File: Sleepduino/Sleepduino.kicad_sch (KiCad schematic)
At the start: 17 parts, among them J1 Barrel_Jack_Switch, J2 Conn_02x03_Counter_Clockwise, U1 ATmega328P-A, U2 ATmega16U2-A, U3 LP2985-3.3, U4 NCP1117-12_TO252, U5 RP2040, Y1 Crystal, Y2 Crystal

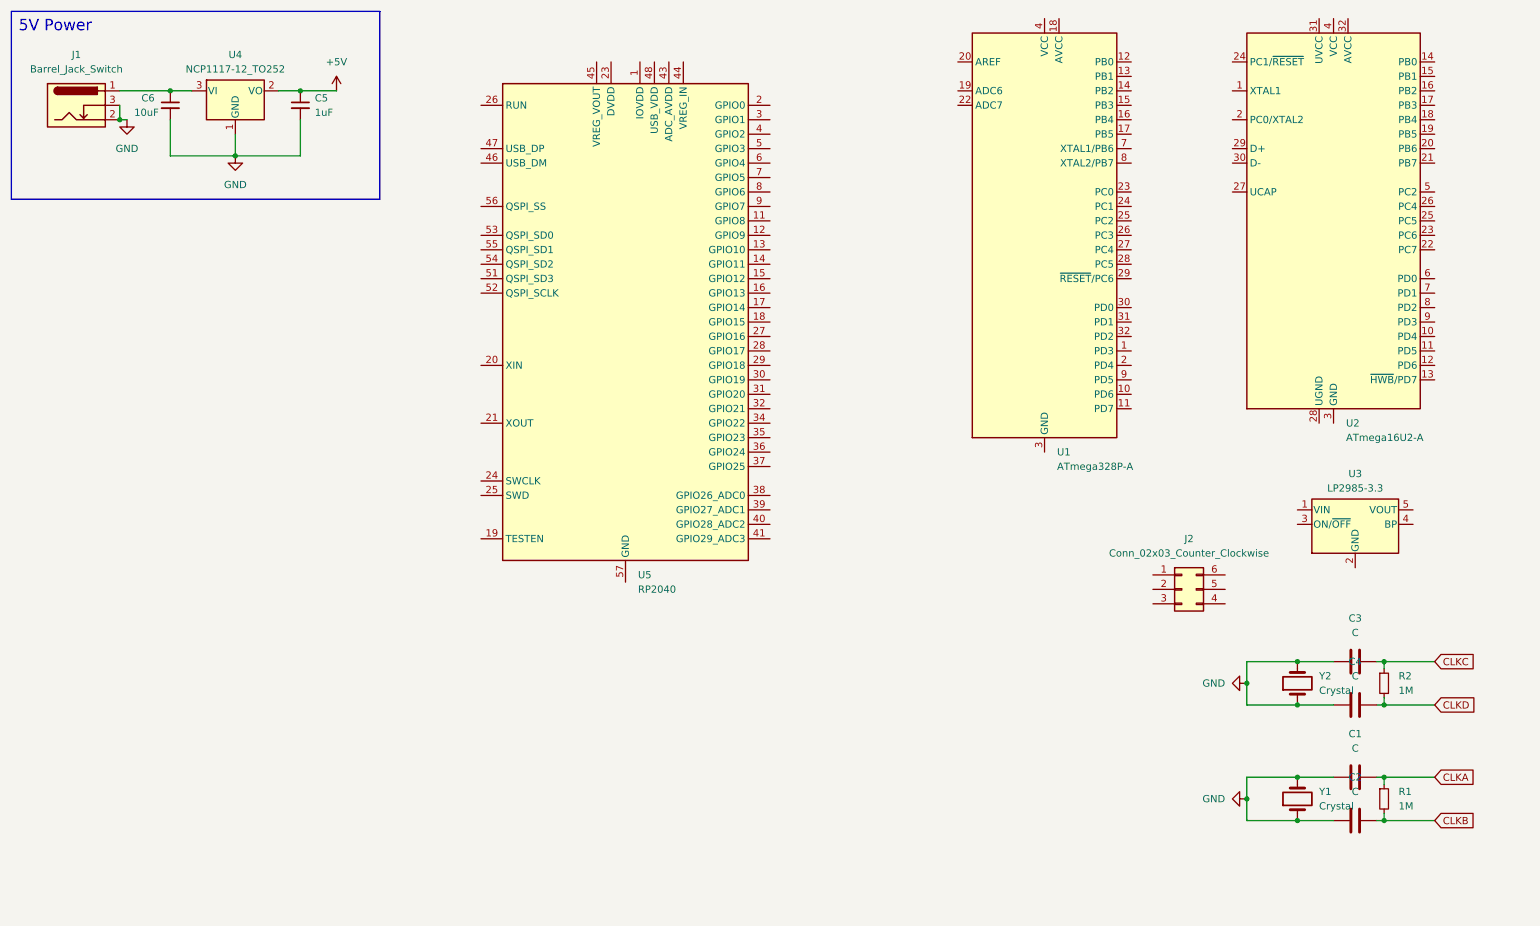
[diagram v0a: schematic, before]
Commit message: massive gains
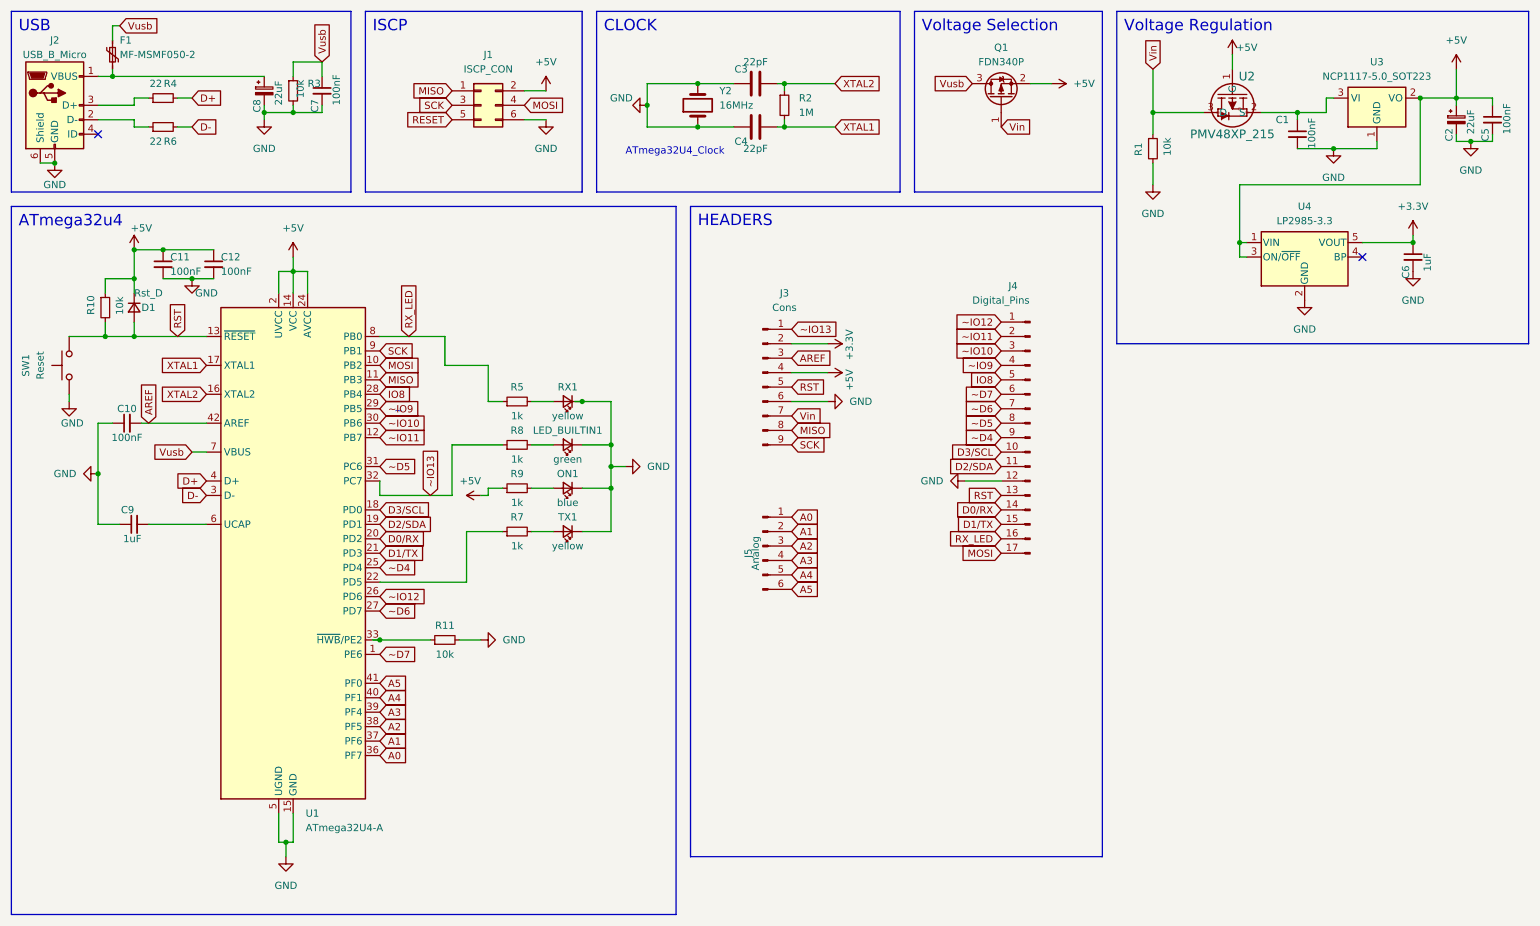
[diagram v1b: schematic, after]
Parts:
- removed C1, C2: C, Capacitor_SMD:C_0402_1005Metric, symbol Device:C
- removed J1: Barrel_Jack_Switch, symbol Connector:Barrel_Jack_Switch
- removed J2: Conn_02x03_Counter_Clockwise, symbol Connector_Generic:Conn_02x03_Counter_Clockwise
- removed U1: ATmega328P-A, Package_QFP:TQFP-32_7x7mm_P0.8mm, symbol MCU_Microchip_ATmega:ATmega328P-A
- removed U2: ATmega16U2-A, Package_QFP:TQFP-32_7x7mm_P0.8mm, symbol MCU_Microchip_ATmega:ATmega16U2-A
- removed U3: LP2985-3.3, Package_TO_SOT_SMD:SOT-23-5, symbol Regulator_Linear:LP2985-3.3
- removed U4: NCP1117-12_TO252, Package_TO_SOT_SMD:TO-252-2, symbol Regulator_Linear:NCP1117-12_TO252
- removed U5: RP2040, Package_DFN_QFN:QFN-56-1EP_7x7mm_P0.4mm_EP3.2x3.2mm, symbol MCU_RaspberryPi:RP2040
- removed Y1: Crystal, Crystal:Crystal_HC49-4H_Vertical, symbol Device:Crystal
- added C1, C10, C11, C12, C7: 100nF, Capacitor_SMD:C_0402_1005Metric, symbol Device:C_Small
- added C2, C8: 22uF, Capacitor_SMD:C_0402_1005Metric, symbol Device:C_Polarized_Small
- added C9: 1uF, Capacitor_SMD:C_0402_1005Metric, symbol Device:C_Small
- added D1: Rst_D, Diode_SMD:D_SOD-323, symbol Device:D_Small
- added F1: MF-MSMF050-2, Fuse:Fuse_1812_4532Metric, symbol Device:Polyfuse_Small
- added J1: ISCP_CON, Connector_PinHeader_2.54mm:PinHeader_2x03_P2.54mm_Vertical, symbol Connector_Generic:Conn_02x03_Odd_Even
- added J2: USB_B_Micro, Connector_USB:USB_Micro-B_Molex-105017-0001, symbol Connector:USB_B_Micro
- added J3: Cons, Connector_PinHeader_2.54mm:PinHeader_1x09_P2.54mm_Vertical, symbol Connector:Conn_01x09_Pin
- added J4: Digital_Pins, Connector_PinHeader_2.54mm:PinHeader_1x17_P2.54mm_Vertical, symbol Connector:Conn_01x17_Pin
- added J5: Analog, Connector_PinHeader_2.54mm:PinHeader_1x06_P2.54mm_Vertical, symbol Connector:Conn_01x06_Pin
- added LED_BUILTIN1: green, LED_SMD:LED_0603_1608Metric, symbol Device:LED_Small
- added ON1: blue, LED_SMD:LED_0603_1608Metric, symbol Device:LED_Small
- added Q1: FDN340P, Package_TO_SOT_SMD:SOT-23, symbol Transistor_FET:FDN340P
- added R10, R11, R3: 10k, Resistor_SMD:R_0402_1005Metric, symbol Device:R_Small
- added R4, R6: 22, Resistor_SMD:R_0402_1005Metric, symbol Device:R_Small
- added R5, R7, R8, R9: 1k, Resistor_SMD:R_0402_1005Metric, symbol Device:R_Small
- added RX1, TX1: yellow, LED_SMD:LED_0603_1608Metric, symbol Device:LED_Small
- added SW1: Reset, Button_Switch_SMD:SW_SPST_TL3342, symbol Switch:SW_Push
- added U1: ATmega32U4-A, Package_QFP:TQFP-44_10x10mm_P0.8mm, symbol MCU_Microchip_ATmega:ATmega32U4-A
- added U2: PMV48XP_215, footprints:TO-236_SOT23_NEX, symbol 2023-11-08_00-09-48:PMV48XP_215
- added U3: NCP1117-5.0_SOT223, Package_TO_SOT_SMD:SOT-223-3_TabPin2, symbol Regulator_Linear:NCP1117-5.0_SOT223
- added U4: LP2985-3.3, Package_TO_SOT_SMD:SOT-23-5, symbol Regulator_Linear:LP2985-3.3
- C3, C4: value C -> 22pF
- C5: value 1uF -> 100nF; footprint (none) -> Capacitor_SMD:C_0402_1005Metric
- C6: value 10uF -> 1uF; footprint (none) -> Capacitor_SMD:C_0402_1005Metric
- R1: value 1M -> 10k
- Y2: value Crystal -> 16MHz
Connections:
- net CLKB is gone; now on net GND: R1.2
- net +5V: now also C11.1, C12.1, C2.1, D1.1 (K), J1.2 (Pin_2), J3.4 (Pin_4), Q1.2 (S), R10.1, R9.1, U1.14 (VCC), U1.2 (UVCC), U1.24 (AVCC), U1.34 (VCC), U1.44 (AVCC), U2.1 (G), U3.2 (VO), U4.1 (VIN), U4.3 (ON/~{OFF})
- net GND: now also C1.2, C10.1, C11.2, C12.2, C2.2, C7.2, C8.2, C9.1, J1.6 (Pin_6), J2.5 (GND), J2.6 (Shield), J3.6 (Pin_6), J4.12 (Pin_12), LED_BUILTIN1.1 (K), ON1.1 (K), R11.2, R3.2, RX1.1 (K), SW1.1, TX1.1 (K), U1.15 (GND), U1.23 (GND), U1.35 (GND), U1.43 (GND), U1.5 (UGND), U3.1 (GND), U4.2 (GND)
- net +3.3V: now reaches C6.1
- net +3.3V: now also J3.2 (Pin_2), U4.5 (VOUT)
- net CLKA renamed Vin
- net Vin: now also J3.7 (Pin_7), Q1.1 (G), U2.3 (D)
- net CLKC renamed XTAL2
- net XTAL2: now also U1.16 (XTAL2)
- net CLKD renamed XTAL1
- net XTAL1: now also U1.17 (XTAL1)
- new net: R7.1, U1.22 (PD5)
- new net: R11.1, U1.33 (~{HWB}/PE2)
- new net: C9.2, U1.6 (UCAP)
- new net: C1.1, U2.2 (S), U3.3 (VI)
- new net: J2.3 (D+), R4.1
- new net: LED_BUILTIN1.2 (A), R8.2
- new net: R5.2, RX1.2 (A)
- new net: C8.1, F1.2, J2.1 (VBUS)
- new net: R7.2, TX1.2 (A)
- new net: J2.2 (D-), R6.1
- new net: ON1.2 (A), R9.2
- new net A0: J5.1 (Pin_1), U1.36 (PF7)
- new net A1: J5.2 (Pin_2), U1.37 (PF6)
- new net A2: J5.3 (Pin_3), U1.38 (PF5)
- new net A3: J5.4 (Pin_4), U1.39 (PF4)
- new net A4: J5.5 (Pin_5), U1.40 (PF1)
- new net A5: J5.6 (Pin_6), U1.41 (PF0)
- new net AREF: C10.2, J3.3 (Pin_3), U1.42 (AREF)
- new net D+: R4.2, U1.4 (D+)
- new net D-: R6.2, U1.3 (D-)
- new net D0/RX: J4.14 (Pin_14), U1.20 (PD2)
- new net D1/TX: J4.15 (Pin_15), U1.21 (PD3)
- new net D2/SDA: J4.11 (Pin_11), U1.19 (PD1)
- new net D3/SCL: J4.10 (Pin_10), U1.18 (PD0)
- new net IO8: J4.5 (Pin_5), U1.28 (PB4)
- new net MISO: J1.1 (Pin_1), J3.8 (Pin_8), U1.11 (PB3)
- new net MOSI: J1.4 (Pin_4), J4.17 (Pin_17), U1.10 (PB2)
- new net RESET: J1.5 (Pin_5)
- new net RST: D1.2 (A), J3.5 (Pin_5), J4.13 (Pin_13), R10.2, SW1.2, U1.13 (~{RESET})
- new net RX_LED: J4.16 (Pin_16), R5.1, U1.8 (PB0)
- new net SCK: J1.3 (Pin_3), J3.9 (Pin_9), U1.9 (PB1)
- new net Vusb: C7.1, F1.1, Q1.3 (D), R3.1, U1.7 (VBUS)
- new net ~D4: J4.9 (Pin_9), U1.25 (PD4)
- new net ~D5: J4.8 (Pin_8), U1.31 (PC6)
- new net ~D6: J4.7 (Pin_7), U1.27 (PD7)
- new net ~D7: J4.6 (Pin_6), U1.1 (PE6)
- new net ~IO10: J4.3 (Pin_3), U1.30 (PB6)
- new net ~IO11: J4.2 (Pin_2), U1.12 (PB7)
- new net ~IO12: J4.1 (Pin_1), U1.26 (PD6)
- new net ~IO13: J3.1 (Pin_1), R8.1, U1.32 (PC7)
- new net ~IO9: J4.4 (Pin_4), U1.29 (PB5)
- no-connect marks 0 -> 2
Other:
- note added: "ATmega32U4_Clock"
- note added: "ATmega32u4"
- note added: "CLOCK"
- note added: "HEADERS"
- note added: "ISCP"
- note added: "USB"
- note added: "Voltage Regulation"
- note added: "Voltage Selection"
- note added: "~"
- note removed: "5V Power"
- moved on the sheet: C3, C4, R2, Y2
